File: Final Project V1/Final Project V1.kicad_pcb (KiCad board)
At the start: 2 copper layers, 67.4 x 68 mm, 46 parts, among them J1 39299043, J2 Conn_02x03_Counter_Clockwise, J3 Conn_02x02_Counter_Clockwise, J4 Conn_02x01, J5 Conn_02x01, J6 Conn_02x09_Counter_Clockwise, J7 Conn_02x01, Q1 SS8050-G, Q2 SS8050-G, SW3 1825910-6, SW4 SW_Wuerth_450301014042, SW5 SW_Wuerth_450301014042, SW6 1825910-6, U1 AP2112K-3.3, U2 ESP32-S3-WROOM-1, U3 BQ21040DBVR, U4 2SJ652-1E, U5 2SJ652-1E

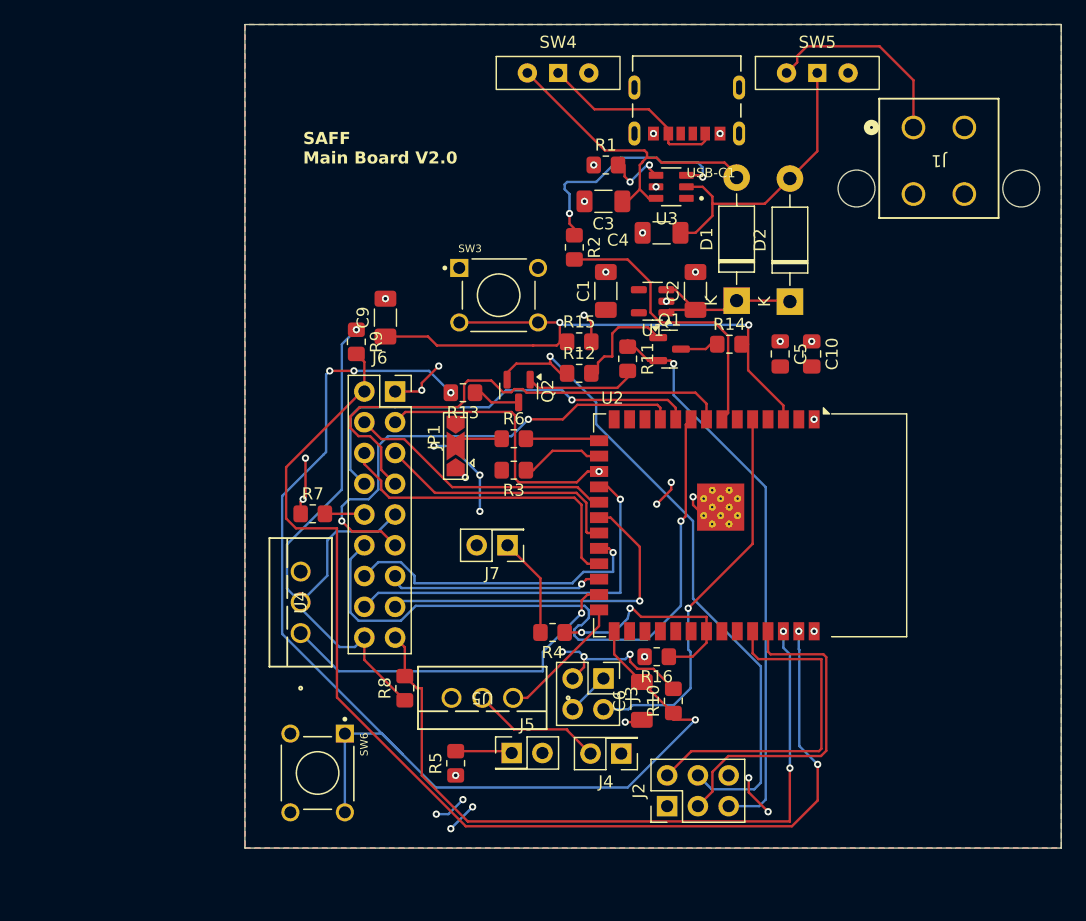
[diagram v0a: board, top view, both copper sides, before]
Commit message: V2 Board
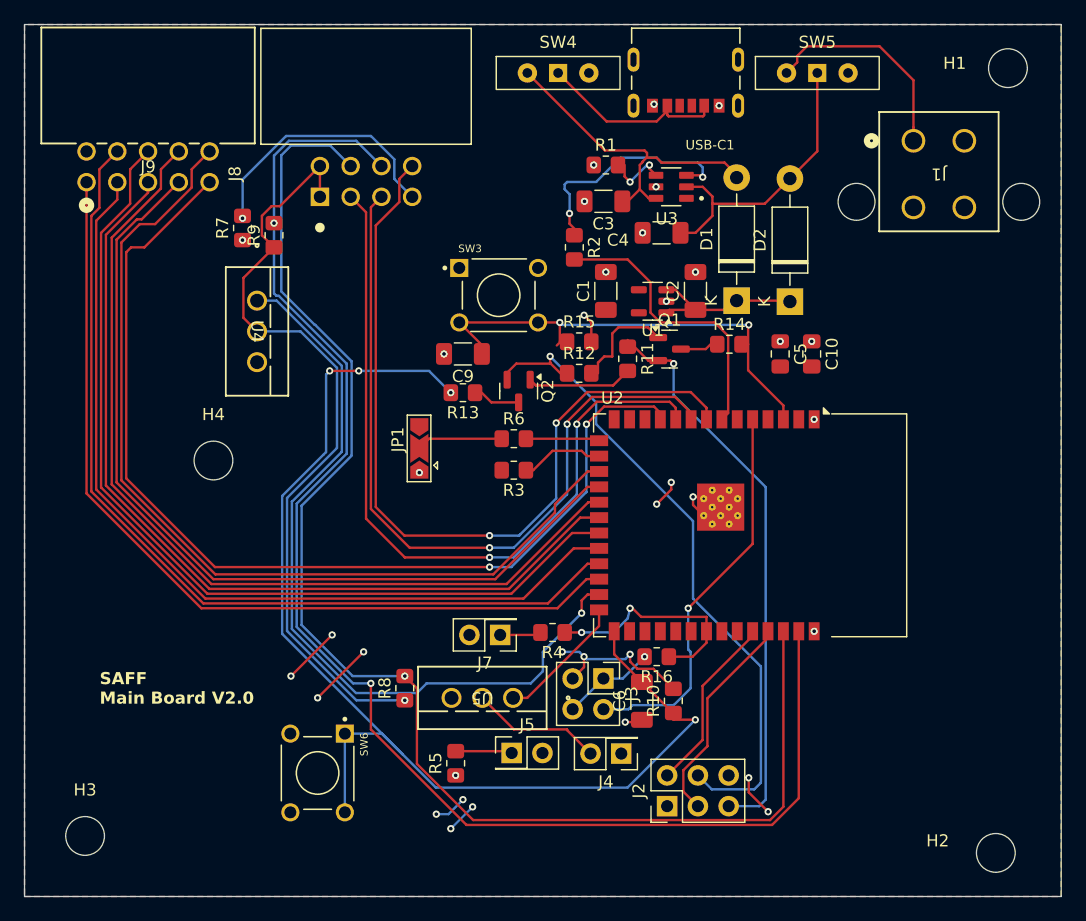
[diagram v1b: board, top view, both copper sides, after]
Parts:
- removed J6: Conn_02x09_Counter_Clockwise, Connector_PinSocket_2.54mm:PinSocket_2x09_P2.54mm_Vertical
- added H1: MountingHoleM3, MountingHole:MountingHole_3.2mm_M3_DIN965, F.Cu at (227.0, 72.2)
- added H2: MountingHoleM3, MountingHole:MountingHole_3.2mm_M3_DIN965, F.Cu at (226.0, 137.0)
- added H3: MountingHoleM3, MountingHole:MountingHole_3.2mm_M3_DIN965, F.Cu at (150.8, 135.6)
- added H4: MountingHoleM3, MountingHole:MountingHole_3.2mm_M3_DIN965, F.Cu at (161.4, 104.6)
- added J8: 75867-132LF, 75867_132LF:HDRRA8W62P254_4X2_1737X957H920, F.Cu at (174.0, 81.6)
- added J9: 10056845-110LF, 75867-101LF:CON10_2X5_R2_FCI_GLE, F.Cu at (150.9, 81.6)
- moved U4 27.7 mm to (165.0, 91.4), turned to -90 degrees
- moved R7 24.3 mm to (163.8, 85.4), turned to 90 degrees
- moved R9 11.1 mm to (166.4, 86.0), turned to 90 degrees
- moved J7 7.42 mm to (185.1, 119.0)
- moved C9 7.07 mm to (182.0, 95.8), turned to 180 degrees
- moved JP1 3.01 mm to (178.4, 103.6)
- moved USB-C1 2.30 mm to (200.4, 75.3)
- moved J1 1.10 mm to (219.2, 78.2)
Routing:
- net D7: track 21.0 -> 76.2 mm
- net D4: track 17.9 -> 72.9 mm, vias 1 -> 0
- net PCLK: track 22.1 -> 76.8 mm
- net VS: track 23.0 -> 77.5 mm, vias 1 -> 0
- net SDA: track 60.4 -> 114.7 mm, vias 2 -> 1
- net D5: track 26.7 -> 76.1 mm
- net D6: track 25.4 -> 73.1 mm, vias 1 -> 0
- net D0: track 39.4 -> 84.6 mm
- net MCLK: track 29.2 -> 73.2 mm, vias 1 -> 0
- net HS: track 31.5 -> 73.5 mm, vias 1 -> 0
- net Camera Power Signal: track 30.1 -> 65.1 mm
- net D1: track 35.3 -> 64.0 mm, vias 1 -> 2
- net D3: track 41.4 -> 68.2 mm, vias 0 -> 2
- net SCL: track 94.9 -> 118.6 mm
- net Net-(J8-Pad7): track 3.28 -> 21.7 mm, vias 0 -> 1
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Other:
- board size 67.4 x 68 mm -> 85.6 x 72 mm
